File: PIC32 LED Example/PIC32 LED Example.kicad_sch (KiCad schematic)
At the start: 18 parts, among them J1 Conn_01x02, J2 Conn_01x05, J3 Conn_01x02_Pin, U1 PIC32MX575F256H, U2 AMS1117-3.3

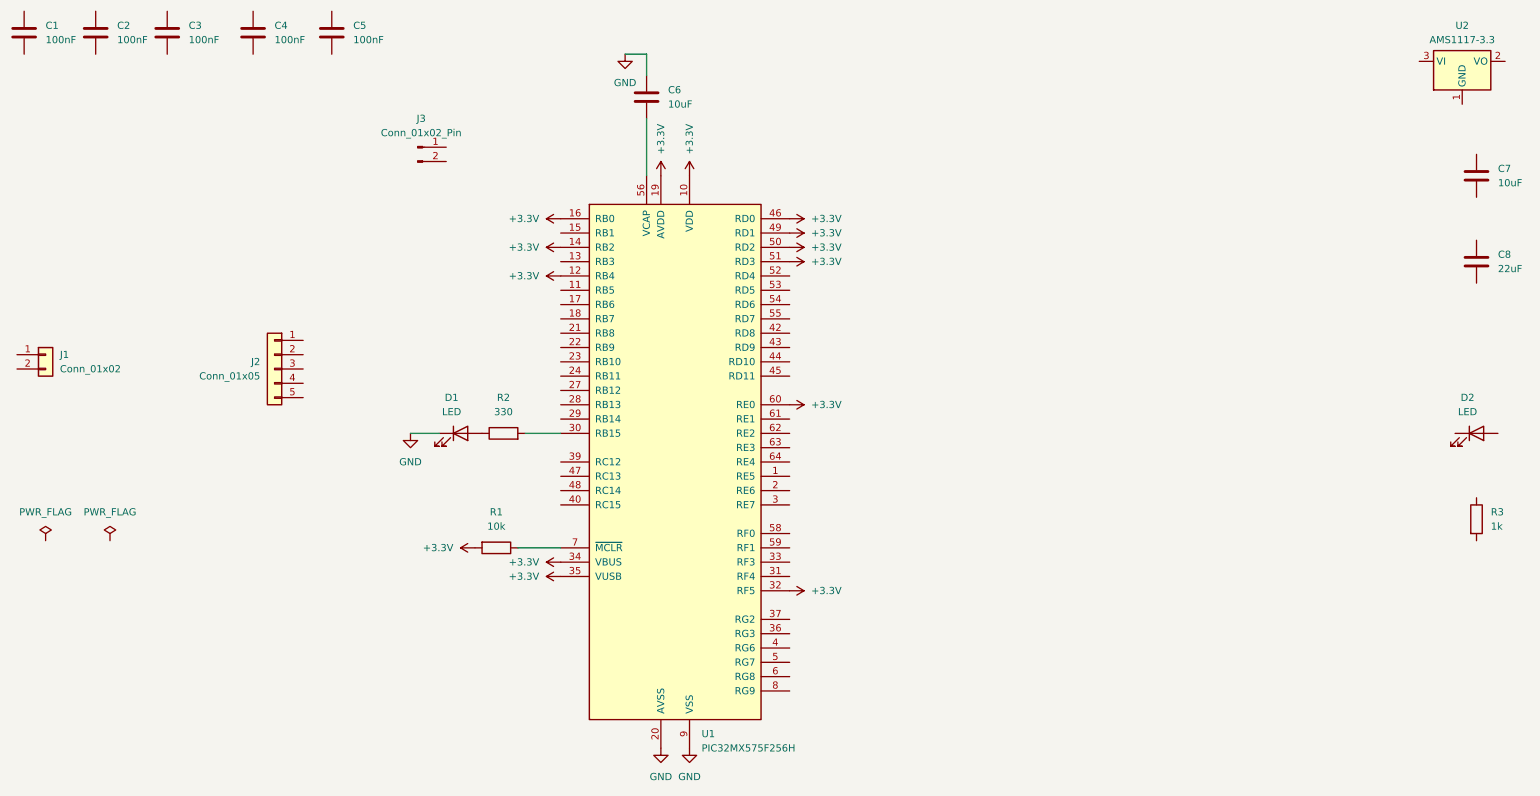
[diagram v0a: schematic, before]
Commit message: finished ERC approved PIC32 LED example
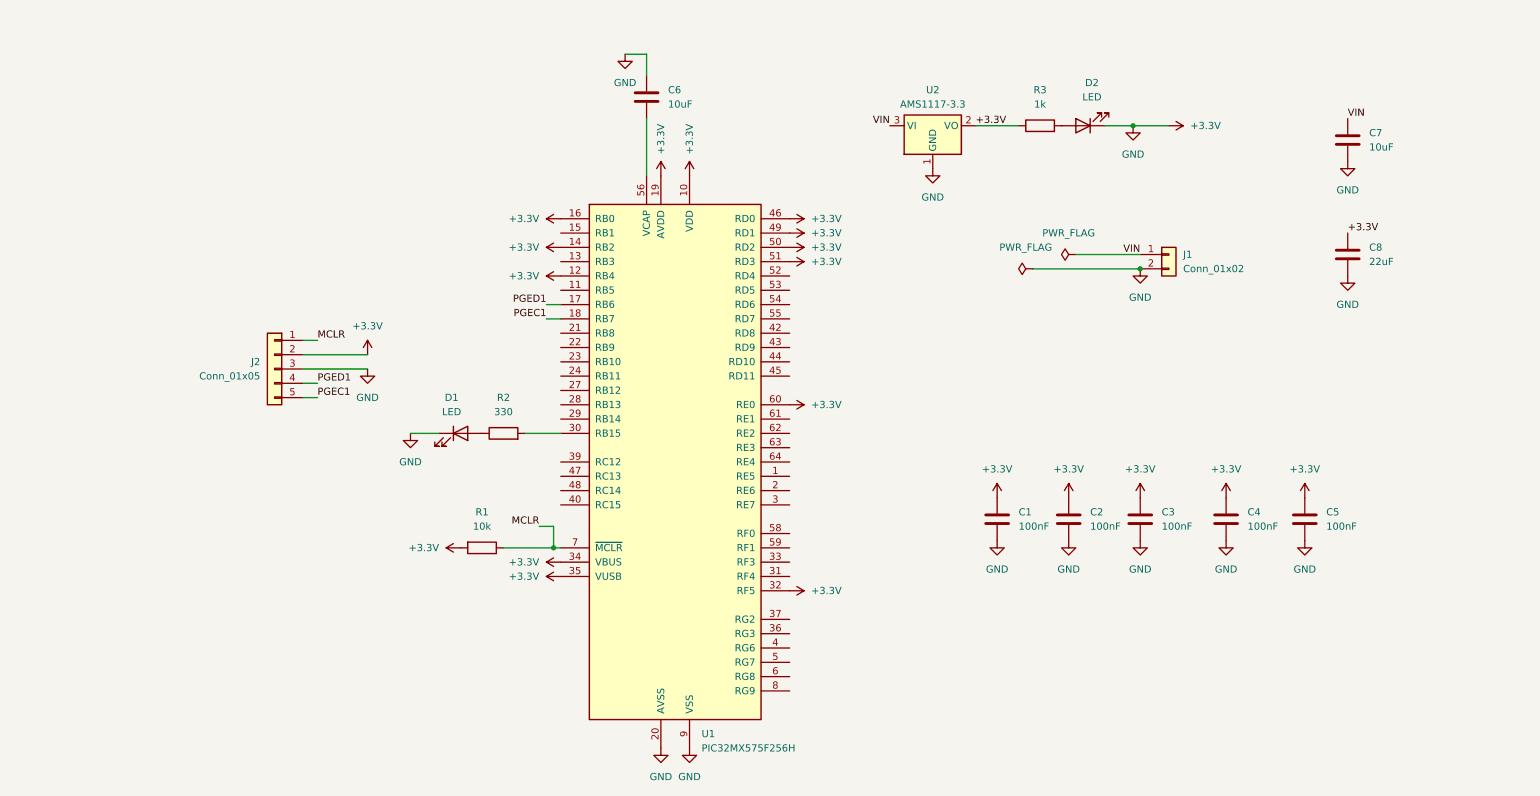
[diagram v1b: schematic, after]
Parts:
- removed J3: Conn_01x02_Pin, symbol Connector:Conn_01x02_Pin
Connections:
- net GND is gone; now on net +3.3V: C6.1, D1.1 (K), U1.20 (AVSS), U1.25 (VSS), U1.41 (VSS), U1.9 (VSS)
- net +3.3V: now also C1.1, C1.2, C2.1, C2.2, C3.1, C3.2, C4.1, C4.2, C5.1, C5.2, C7.2, C8.1, C8.2, D2.1 (K), J1.2 (Pin_2), J2.2 (Pin_2), J2.3 (Pin_3), R3.1, U2.1 (GND), U2.2 (VO)
- net VIN: now reaches J1.1 (Pin_1)
- net VIN: now also C7.1, U2.3 (VI)
- net at D2.2 (A): now also R3.2
- net MCLR: now reaches R1.1, U1.7 (~{MCLR})
- net MCLR: now also J2.1 (Pin_1)
- net PGED1: now reaches U1.17 (RB6)
- net PGED1: now also J2.4 (Pin_4)
- net PGEC1: now reaches U1.18 (RB7)
- net PGEC1: now also J2.5 (Pin_5)
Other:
- moved on the sheet: C1, C2, C3, C4, C5, C7, C8, D2, J1, R1, R3, U2
